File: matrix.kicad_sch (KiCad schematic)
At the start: 94 parts, among them SW10 K08, SW11 K09, SW12 K0A, SW13 K0B, SW14 K0C, SW15 K10, SW16 K11, SW17 K12, SW18 K13, SW19 K14, SW2 K00, SW20 K15, SW21 K16, SW22 K17, SW23 K18, SW24 K19, SW25 K1A, SW26 K1B, SW27 K20, SW28 K21, SW29 K22, SW3 K01, SW30 K23, SW31 K24, SW32 K25, SW33 K26, SW34 K27, SW35 K28, SW36 K29, SW37 K2A, SW38 K2B, SW39 K30, SW4 K02, SW40 K31, SW41 K32, SW42 K33, SW43 K34, SW44 K36, SW45 K38, SW46 K39, SW47 K3A, SW48 K3B, SW5 K03, SW6 K04, SW7 K05, SW8 K06, SW9 K07

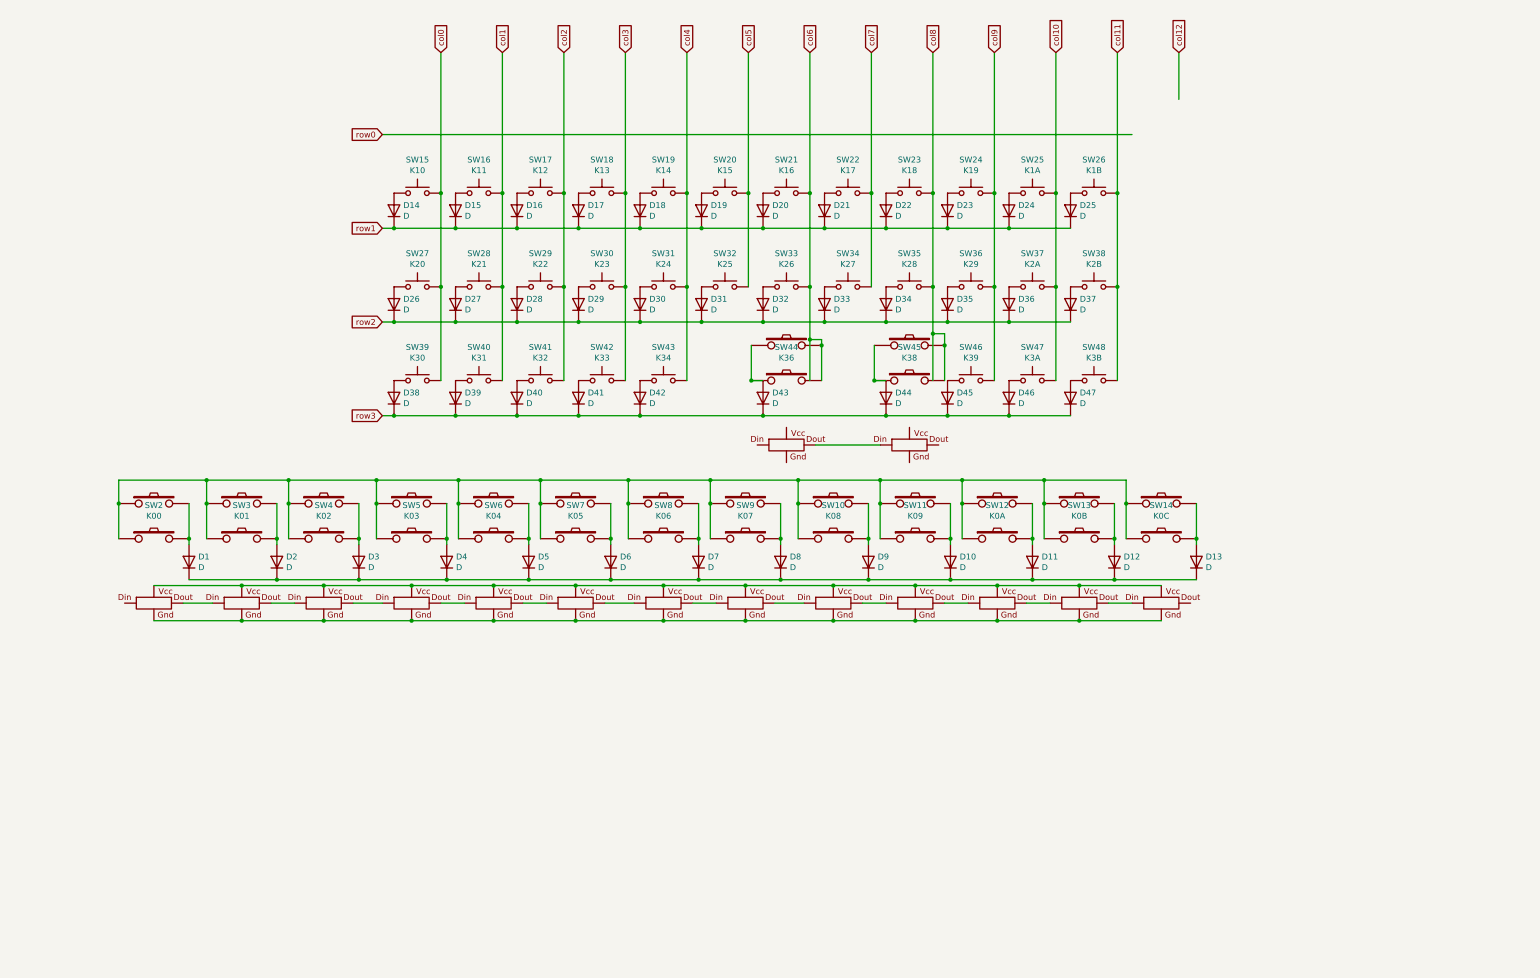
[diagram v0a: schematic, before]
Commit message: 2d line on schem
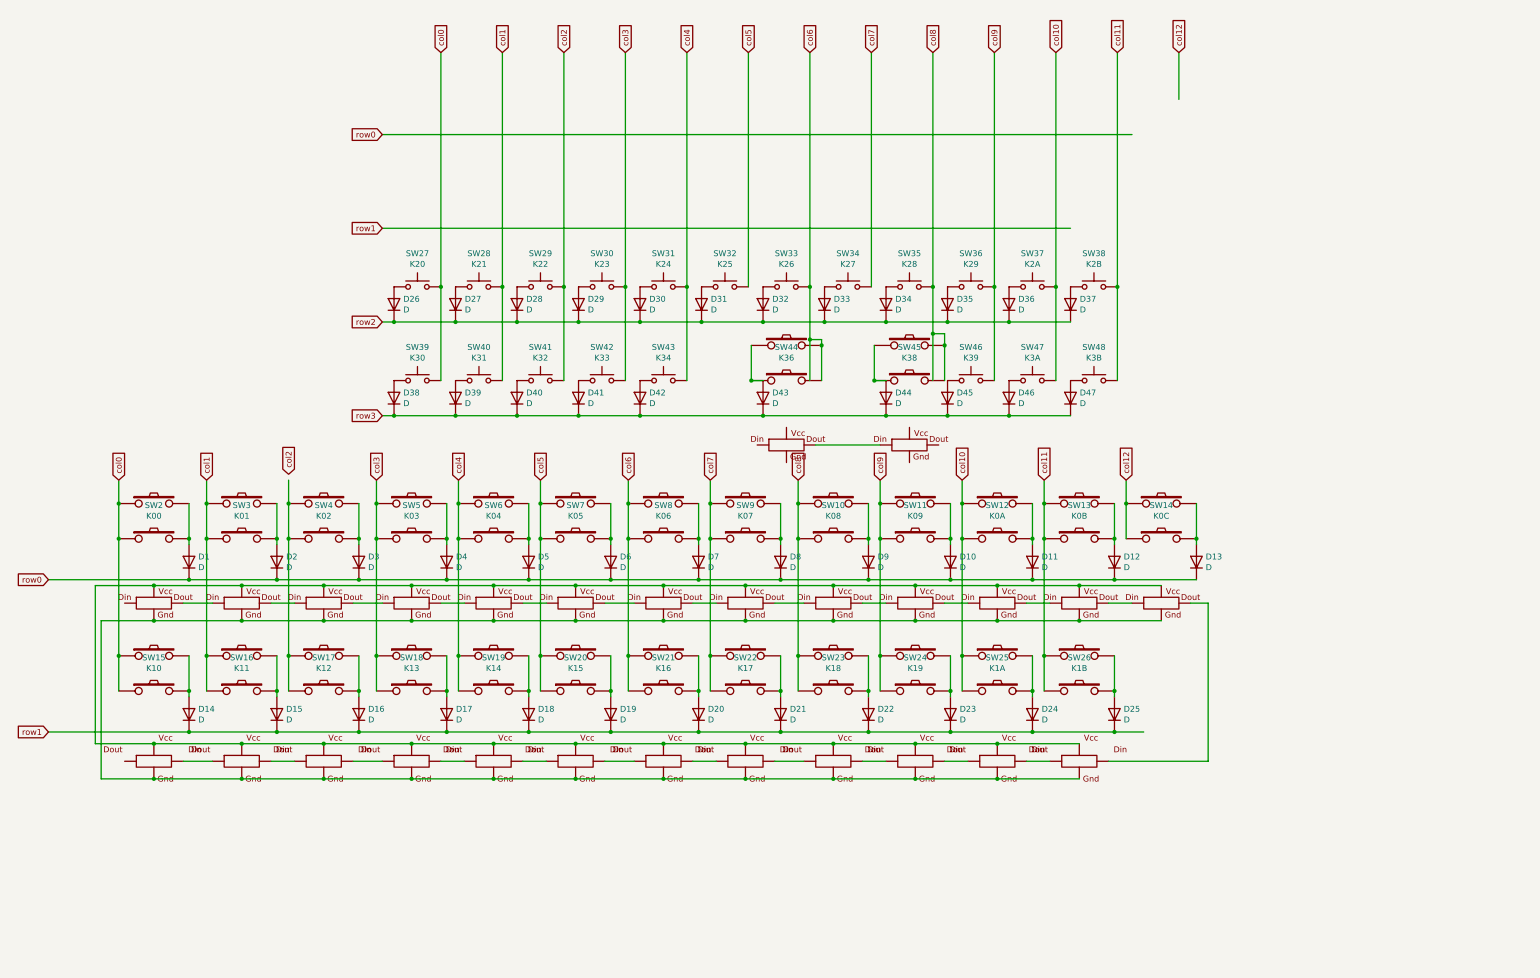
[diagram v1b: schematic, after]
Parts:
- SW15, SW16, SW17, SW18, SW19, SW20, SW21, SW22, SW23, SW24, SW25, SW26: symbol Switch:SW_Push -> switches:SWITCH_PUSH_MXCHOC_REVERSELED
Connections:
- net col0: now also SW15.1, SW15.3, SW2.1, SW2.3; no longer SW15.2
- net col1: now also SW16.1, SW16.3, SW3.1, SW3.3; no longer SW16.2
- net col10: now also SW12.1, SW12.3, SW25.1, SW25.3; no longer SW25.2
- net col11: now also SW13.1, SW13.3, SW26.1, SW26.3; no longer SW26.2
- net col12: now also SW14.1, SW14.3
- net col2: no longer SW17.2
- net col3: now also SW18.1, SW18.3, SW5.1, SW5.3; no longer SW18.2
- net col4: now also SW19.1, SW19.3, SW6.1, SW6.3; no longer SW19.2
- net col5: now also SW20.1, SW20.3, SW7.1, SW7.3; no longer SW20.2
- net col6: now also SW21.1, SW21.3, SW8.1, SW8.3; no longer SW21.2
- net col7: now also SW22.1, SW22.3, SW9.1, SW9.3; no longer SW22.2
- net col8: now also SW10.1, SW10.3, SW23.1, SW23.3; no longer SW23.2
- net col9: now also SW11.1, SW11.3, SW24.1, SW24.3; no longer SW24.2
- net row0: now also D1.1 (K), D10.1 (K), D11.1 (K), D12.1 (K), D13.1 (K), D2.1 (K), D3.1 (K), D4.1 (K), D5.1 (K), D6.1 (K), D7.1 (K), D8.1 (K), D9.1 (K)
- net at SW10.10 (Vdd), SW11.10 (Vdd), SW12.10 (Vdd)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: now also SW15.10 (Vdd), SW16.10 (Vdd), SW17.10 (Vdd), SW18.10 (Vdd), SW19.10 (Vdd), SW20.10 (Vdd), SW21.10 (Vdd), SW22.10 (Vdd), SW23.10 (Vdd), SW24.10 (Vdd), SW25.10 (Vdd), SW26.10 (Vdd)
- net at SW10.12 (VSS), SW11.12 (VSS), SW12.12 (VSS)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: now also SW15.12 (VSS), SW16.12 (VSS), SW17.12 (VSS), SW18.12 (VSS), SW19.12 (VSS), SW20.12 (VSS), SW21.12 (VSS), SW22.12 (VSS), SW23.12 (VSS), SW24.12 (VSS), SW25.12 (VSS), SW26.12 (VSS)
- net at SW14.9 (Dout): now also SW26.11 (Din)
- net at SW17.1: now also SW17.3, SW4.1, SW4.3; no longer D16.2 (A)
- net at D17.2 (A): now also SW18.2, SW18.4; no longer SW18.1
- net at D14.2 (A): now also SW15.2, SW15.4; no longer SW15.1
- net at D15.2 (A): now also SW16.2, SW16.4; no longer SW16.1
- net at D20.2 (A): now also SW21.2, SW21.4; no longer SW21.1
- net at D21.2 (A): now also SW22.2, SW22.4; no longer SW22.1
- net at D25.2 (A): now also SW26.2, SW26.4; no longer SW26.1
- net at D19.2 (A): now also SW20.2, SW20.4; no longer SW20.1
- net at D23.2 (A): now also SW24.2, SW24.4; no longer SW24.1
- net at D22.2 (A): now also SW23.2, SW23.4; no longer SW23.1
- net at D18.2 (A): now also SW19.2, SW19.4; no longer SW19.1
- net at D24.2 (A): now also SW25.2, SW25.4; no longer SW25.1
- new net: SW17.11 (Din), SW18.9 (Dout)
- new net: D16.2 (A), SW17.2, SW17.4
- new net: SW16.11 (Din), SW17.9 (Dout)
- new net: SW18.11 (Din), SW19.9 (Dout)
- new net: SW15.11 (Din), SW16.9 (Dout)
- new net: SW21.11 (Din), SW22.9 (Dout)
- new net: SW20.11 (Din), SW21.9 (Dout)
- new net: SW22.11 (Din), SW23.9 (Dout)
- new net: SW19.11 (Din), SW20.9 (Dout)
- new net: SW23.11 (Din), SW24.9 (Dout)
- new net: SW25.11 (Din), SW26.9 (Dout)
- new net: SW24.11 (Din), SW25.9 (Dout)
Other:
- moved on the sheet: D14, D15, D16, D17, D18, D19, D20, D21, D22, D23, D24, D25

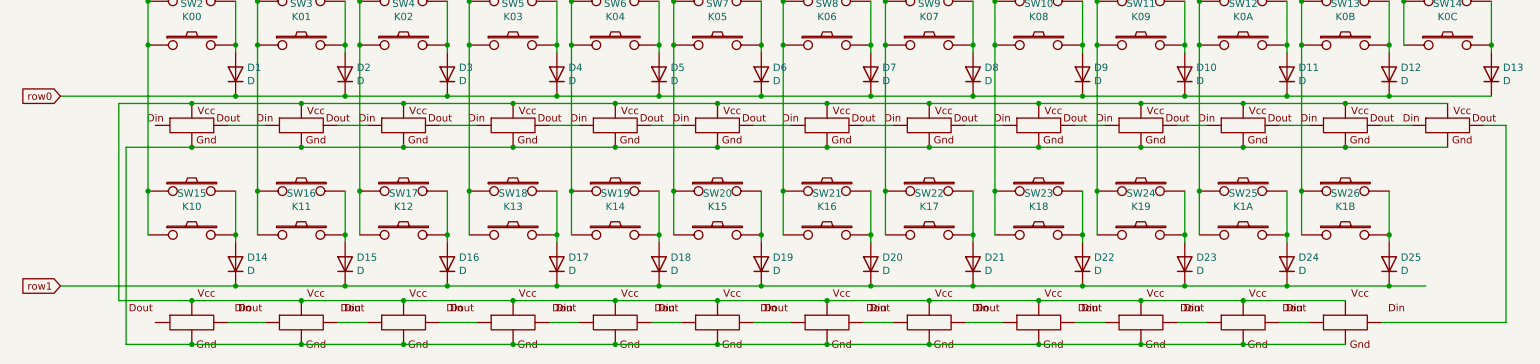
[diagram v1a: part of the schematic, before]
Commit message: moar routing
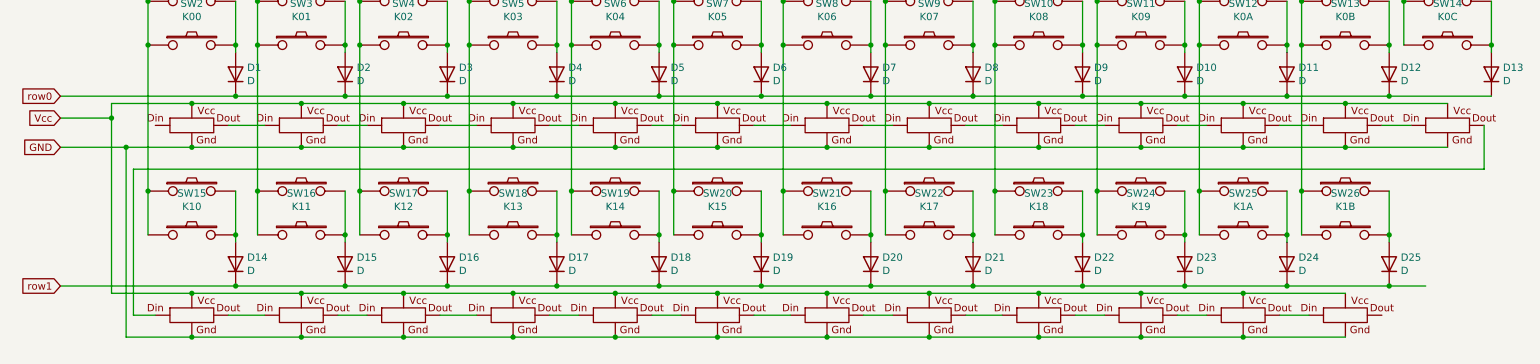
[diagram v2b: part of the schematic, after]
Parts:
- SW15, SW16, SW17, SW18, SW19, SW20, SW21, SW22, SW23, SW24, SW25, SW26: symbol switches:SWITCH_PUSH_MXCHOC_REVERSELED -> switches:SWITCH_PUSH_MXCHOC
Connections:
- net Vcc: now reaches SW10.10 (Vdd), SW11.10 (Vdd), SW12.10 (Vdd), SW13.10 (Vdd), SW14.10 (Vdd), SW15.10 (Vdd), SW16.10 (Vdd), SW17.10 (Vdd), SW18.10 (Vdd), SW19.10 (Vdd), SW2.10 (Vdd), SW20.10 (Vdd), SW21.10 (Vdd), SW22.10 (Vdd), SW23.10 (Vdd), SW24.10 (Vdd), SW25.10 (Vdd), SW26.10 (Vdd), SW3.10 (Vdd), SW4.10 (Vdd), SW5.10 (Vdd), SW6.10 (Vdd), SW7.10 (Vdd), SW8.10 (Vdd), SW9.10 (Vdd)
- net GND: now reaches SW10.12 (VSS), SW11.12 (VSS), SW12.12 (VSS), SW13.12 (VSS), SW14.12 (VSS), SW15.12 (VSS), SW16.12 (VSS), SW17.12 (VSS), SW18.12 (VSS), SW19.12 (VSS), SW2.12 (VSS), SW20.12 (VSS), SW21.12 (VSS), SW22.12 (VSS), SW23.12 (VSS), SW24.12 (VSS), SW25.12 (VSS), SW26.12 (VSS), SW3.12 (VSS), SW4.12 (VSS), SW5.12 (VSS), SW6.12 (VSS), SW7.12 (VSS), SW8.12 (VSS), SW9.12 (VSS)
- net at SW14.9 (Dout): now also SW15.11 (Din); no longer SW26.11 (Din)
- net at SW17.11 (Din): now also SW16.9 (Dout); no longer SW18.9 (Dout)
- net at SW17.9 (Dout): now also SW18.11 (Din); no longer SW16.11 (Din)
- net at SW19.9 (Dout): now also SW20.11 (Din); no longer SW18.11 (Din)
- net at SW15.9 (Dout): now also SW16.11 (Din)
- net at SW21.11 (Din): now also SW20.9 (Dout); no longer SW22.9 (Dout)
- net at SW21.9 (Dout): now also SW22.11 (Din); no longer SW20.11 (Din)
- net at SW23.9 (Dout): now also SW24.11 (Din); no longer SW22.11 (Din)
- net at SW19.11 (Din): now also SW18.9 (Dout); no longer SW20.9 (Dout)
- net at SW23.11 (Din): now also SW22.9 (Dout); no longer SW24.9 (Dout)
- net at SW26.9 (Dout): no longer SW25.11 (Din)
- net at SW25.9 (Dout): now also SW26.11 (Din); no longer SW24.11 (Din)
- new net: SW24.9 (Dout), SW25.11 (Din)
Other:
- moved on the sheet: SW15, SW16, SW17, SW18, SW19, SW20, SW21, SW22, SW23, SW24, SW25, SW26

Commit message: who needs MCUs anyway
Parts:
- SW39, SW46, SW48: footprint Button_Switch_Keyboard:SW_Cherry_MX_1.00u_PCB -> mx_rgb:ChocMx_Socket
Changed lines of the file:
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@@
     (property "Reference" "SW39" (id 0) (at 41.91 90.551 0))
     (property "Value" "K30" (id 1) (at 41.91 92.8624 0))
-    (property "Footprint" "Button_Switch_Keyboard:SW_Cherry_MX_1.00u_PCB" (id 2) (at 41.91 92.71 0)
+    (property "Footprint" "mx_rgb:ChocMx_Socket" (id 2) (at 41.91 92.71 0)
       (effects (font (size 1.27 1.27)) hide)
     )
@@
     (property "Reference" "SW46" (id 0) (at 161.925 90.551 0))
     (property "Value" "K39" (id 1) (at 161.925 92.8624 0))
-    (property "Footprint" "Button_Switch_Keyboard:SW_Cherry_MX_1.00u_PCB" (id 2) (at 161.925 92.71 0)
+    (property "Footprint" "mx_rgb:ChocMx_Socket" (id 2) (at 161.925 92.71 0)
       (effects (font (size 1.27 1.27)) hide)
     )
@@
     (property "Reference" "SW48" (id 0) (at 188.595 90.551 0))
     (property "Value" "K3B" (id 1) (at 188.595 92.8624 0))
-    (property "Footprint" "Button_Switch_Keyboard:SW_Cherry_MX_1.00u_PCB" (id 2) (at 188.595 92.71 0)
-      (effects (font (size 1.27 1.27)) hide)
-    )
+    (property "Footprint" "mx_rgb:ChocMx_Socket" (id 2) (at 188.595 92.71 0)
+      (effects (font (size 1.27 1.27)) hide)
+    )

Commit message: add socket keep out zones
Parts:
- SW44: footprint mx_rgb:ChocMx_Socket -> mx_rgb:mx_with_stabilizer
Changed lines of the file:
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@@
     (property "Reference" "SW44" (id 0) (at 121.92 90.551 0))
     (property "Value" "K36" (id 1) (at 121.92 92.8624 0))
-    (property "Footprint" "mx_rgb:ChocMx_Socket" (id 2) (at 121.92 92.71 0)
+    (property "Footprint" "mx_rgb:mx_with_stabilizer" (id 2) (at 121.92 92.71 0)
       (effects (font (size 1.27 1.27)) hide)
     )

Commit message: switch to 0603
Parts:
- D1, D10, D11, D12, D13, D14, D15, D16, D17, D18, D19, D2, D20, D21, D22, D23, D24, D25, D26, D27, D28, D29, D3, D30, D31, D32, D33, D34, D35, D36, D37, D38, D39, D4, D40, D41, D42, D43, D44, D45, D46, D47, D5, D6, D7, D8, D9: footprint Diode_SMD:D_SOD-323_HandSoldering -> Diode_SMD:D_0603_1608Metric
